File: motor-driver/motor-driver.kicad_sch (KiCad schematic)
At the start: 2 parts, among them J2 Screw_Terminal_01x08

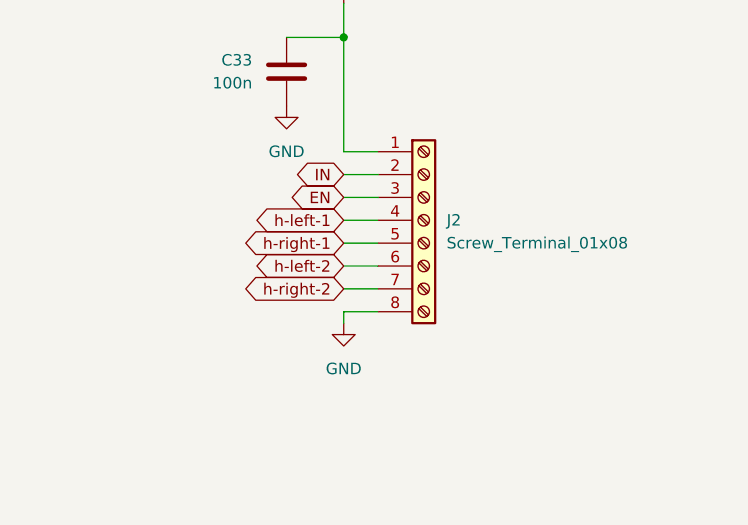
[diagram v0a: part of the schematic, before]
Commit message: pcb layout
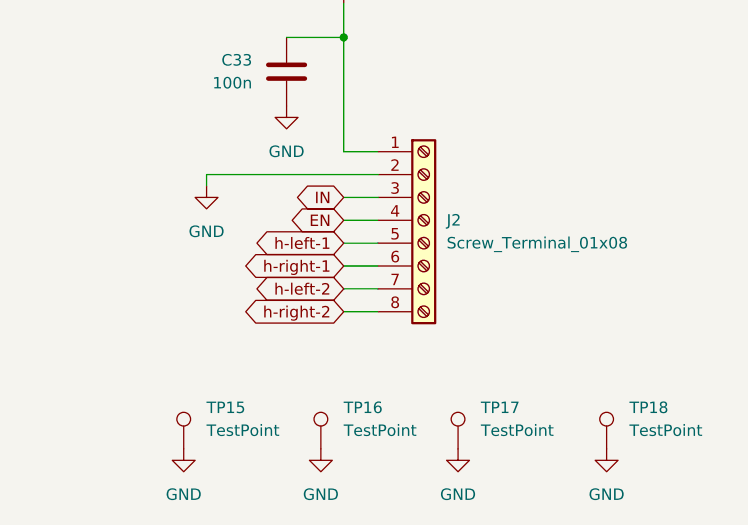
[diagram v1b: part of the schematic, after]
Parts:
- added TP15, TP16, TP17, TP18: TestPoint, TestPoint:TestPoint_Plated_Hole_D3.0mm, symbol Connector:TestPoint
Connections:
- net EN: now also J2.4 (Pin_4); no longer J2.3 (Pin_3)
- net GND: now also J2.2 (Pin_2), TP15.1, TP16.1, TP17.1, TP18.1; no longer J2.8 (Pin_8)
- net IN: now also J2.3 (Pin_3); no longer J2.2 (Pin_2)
- net h-left-1: now also J2.5 (Pin_5); no longer J2.4 (Pin_4)
- net h-left-2: now also J2.7 (Pin_7); no longer J2.6 (Pin_6)
- net h-right-1: now also J2.6 (Pin_6); no longer J2.5 (Pin_5)
- net h-right-2: now also J2.8 (Pin_8); no longer J2.7 (Pin_7)
